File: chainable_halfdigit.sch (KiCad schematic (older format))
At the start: 42 parts, among them J1 Conn_01x03, J2 Conn_01x03

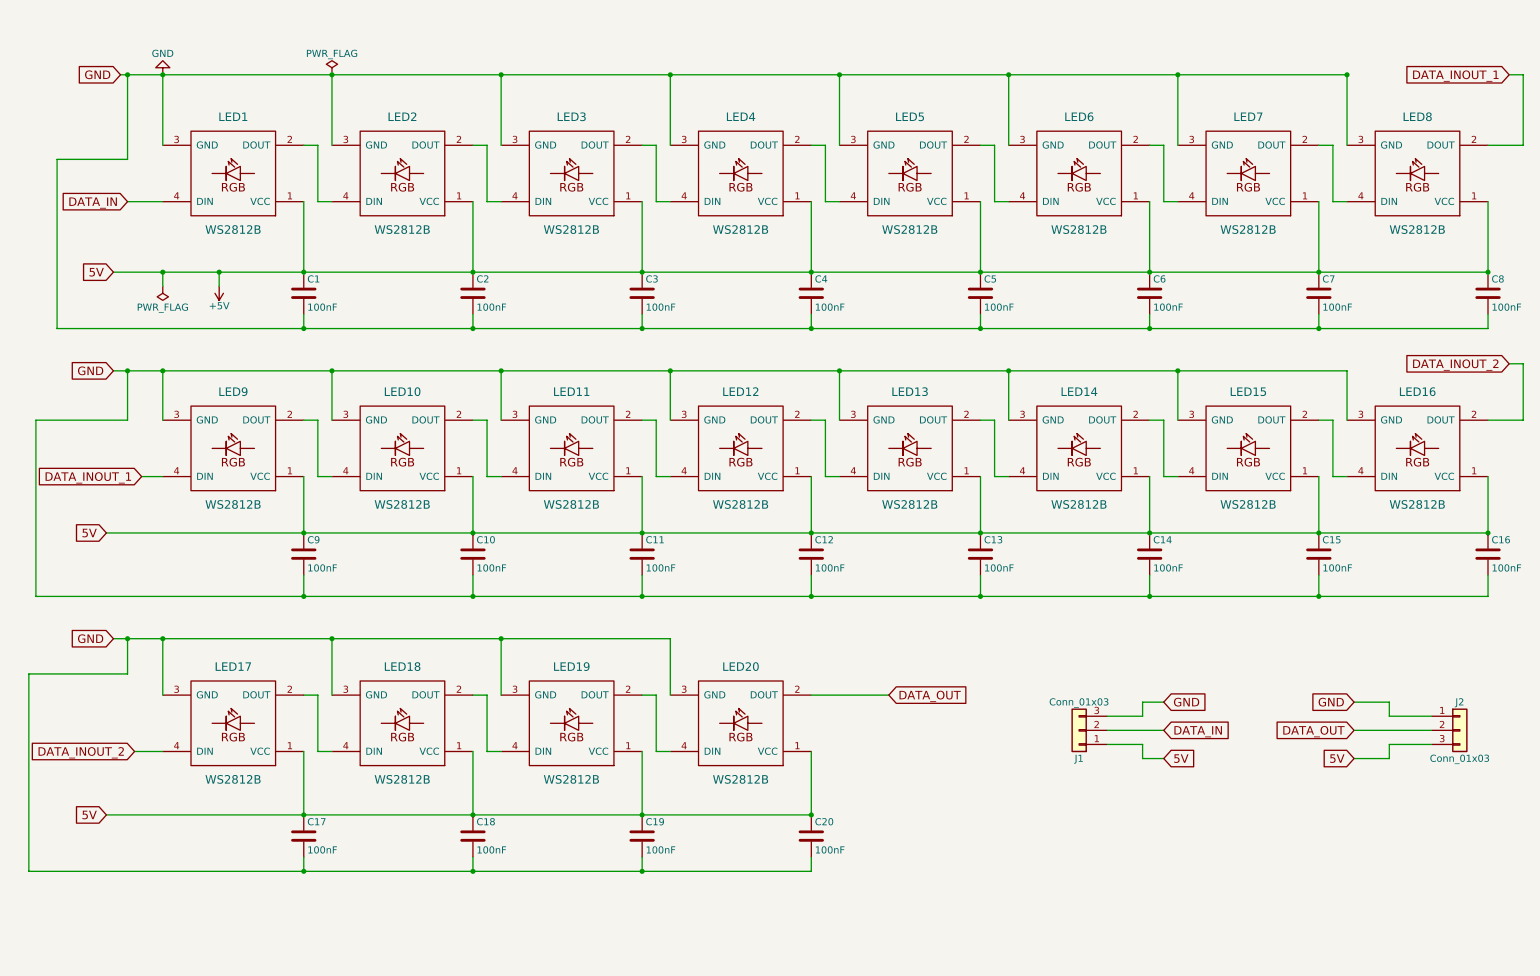
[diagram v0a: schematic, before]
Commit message: Added more LEDs and created PCB
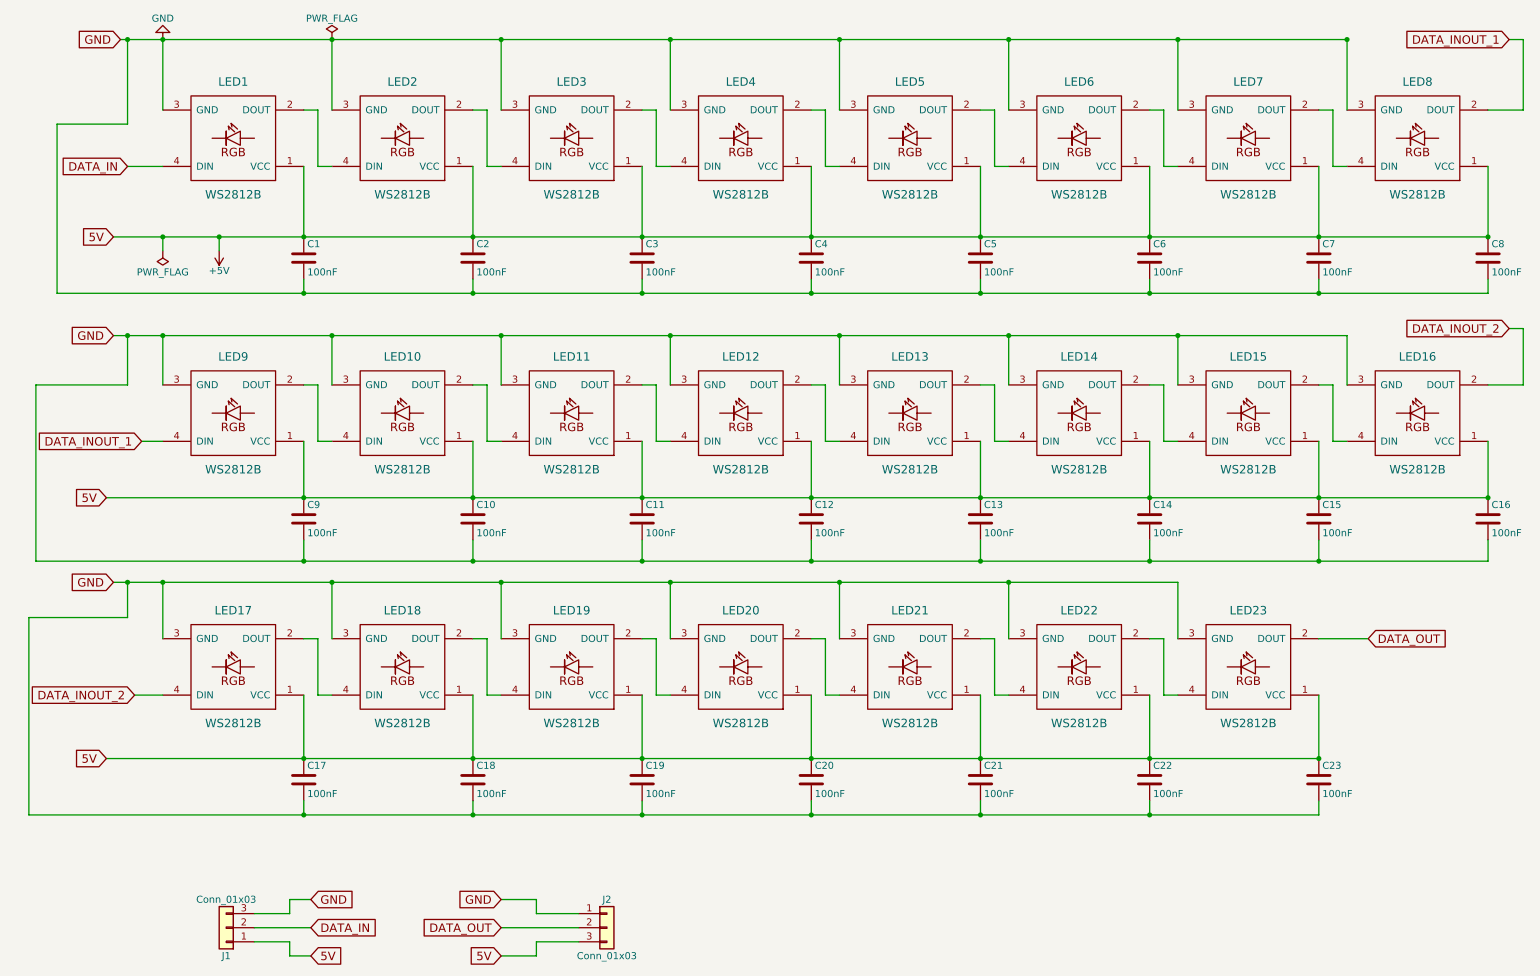
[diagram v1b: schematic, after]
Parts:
- added C21, C22, C23: 100nF, Capacitors_SMD:C_0603, symbol C
- added LED21, LED22, LED23: WS2812B, WS2812B:WS2812B_data-bridgeable, symbol WS2812B
- C1, C10, C11, C12, C13, C14, C15, C16, C17, C18, C19, C2, C20, C3, C4, C5, C6, C7, C8, C9: footprint (none) -> Capacitors_SMD:C_0603
- J1, J2: footprint (none) -> Pin_Headers:Pin_Header_Straight_1x03_Pitch2.54mm
- LED1, LED10, LED11, LED12, LED13, LED14, LED15, LED16, LED17, LED18, LED19, LED2, LED20, LED3, LED4, LED5, LED6, LED7, LED8, LED9: footprint (none) -> WS2812B:WS2812B_data-bridgeable
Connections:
- net +5V: now also C21.1, C22.1, C23.1, LED21.1 (VCC), LED22.1 (VCC), LED23.1 (VCC)
- net DATA_OUT: now also LED23.2 (DOUT); no longer LED20.2 (DOUT)
- net GND: now also C21.2, C22.2, C23.2, LED21.3 (GND), LED22.3 (GND), LED23.3 (GND)
- new net: LED20.2 (DOUT), LED21.4 (DIN)
- new net: LED21.2 (DOUT), LED22.4 (DIN)
- new net: LED22.2 (DOUT), LED23.4 (DIN)
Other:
- moved on the sheet: C1, C10, C11, C12, C13, C14, C15, C16, C17, C18, C19, C2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
